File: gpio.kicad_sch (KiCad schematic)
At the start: 8 parts, among them J1 DF40C-100DP-0.4V(51), J2 DF40C-100DP-0.4V(51), J5 SerDes, U1 LFE5U-85F-6BG381C

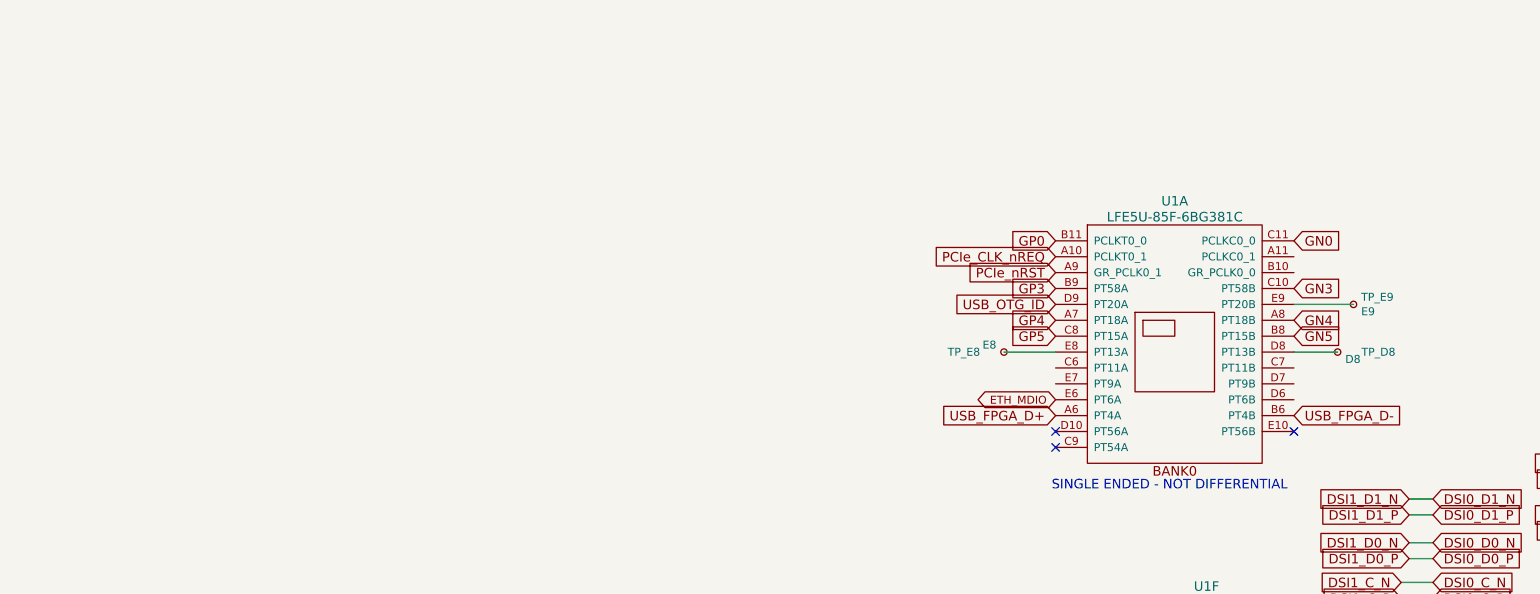
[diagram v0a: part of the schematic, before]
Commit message: Before graphical cleanup
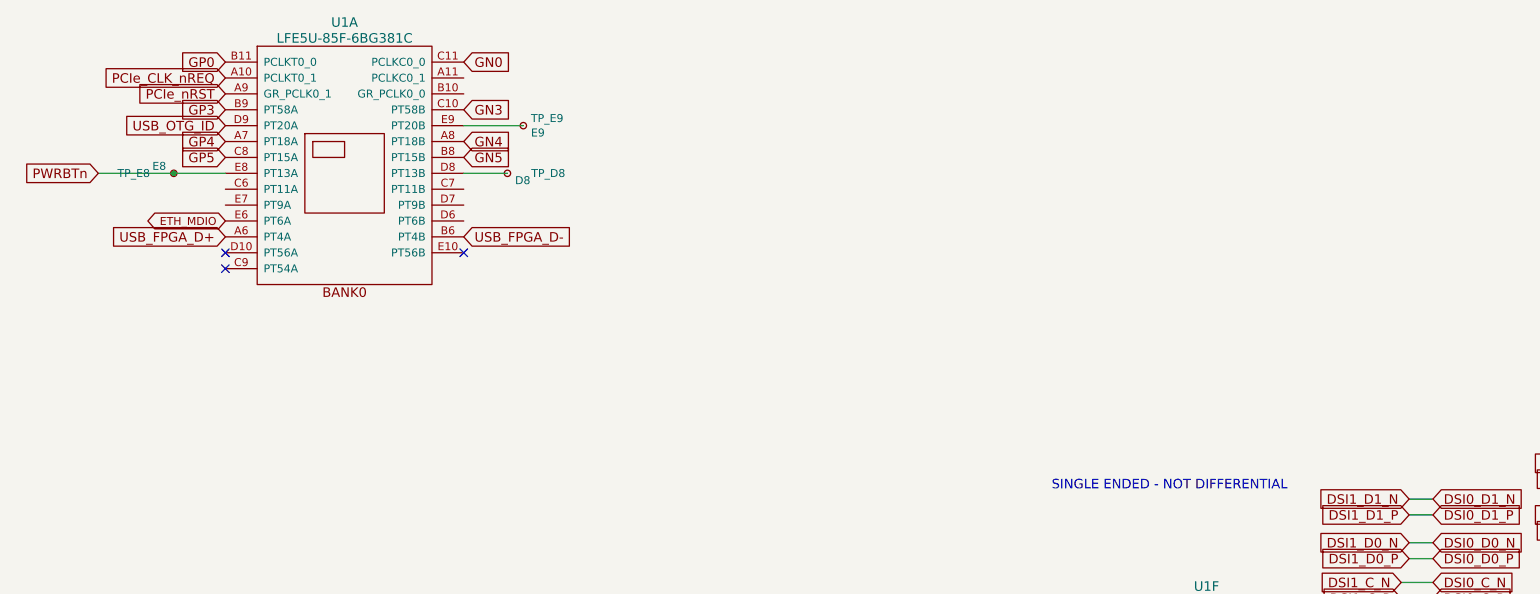
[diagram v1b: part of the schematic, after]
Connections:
- net PWRBTn: now reaches TP_E8.1, U1.E8 (PT13A)
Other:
- moved on the sheet: TP_D8, TP_E8, TP_E9, U1A
